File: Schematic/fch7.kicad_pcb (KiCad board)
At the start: 4 copper layers, 39.8 x 41.5 mm, 144 parts, among them IC1 MP9943AGQ-Z, IC2 MP9943AGQ-Z, IC4 ICM-42688-P, IC5 MPU-6500, J11 PIN2216, J12 PIN2216, J2 PIN2216, J3 PIN2216, J4 PIN2216, J5 PIN2216, J6 PIN2216, J7 PIN2216, J8 PIN2216, J9 PIN2216, U1 ME6217C33M5G, U10 HDGC1002WR-S-4P, U11 HDGC1002WR-S-4P, U12 E28-2G4M27SX, U13 STM32H742VIHx, U15 HDGC1002WR-S-6P, U16 HDGC1002WR-S-8P, U17 HDGC1002WR-S-8P, U2 ME6217C33M5G, U3 LDO-1.8v, U4 QMC5883L, U5 SPL06-001, U6 CSNP1GCR01-BOW, U7 HDGC1002WR-S-6P, U8 HDGC1002WR-S-4P, U9 HDGC1002WR-S-4P, Y1 8MHz

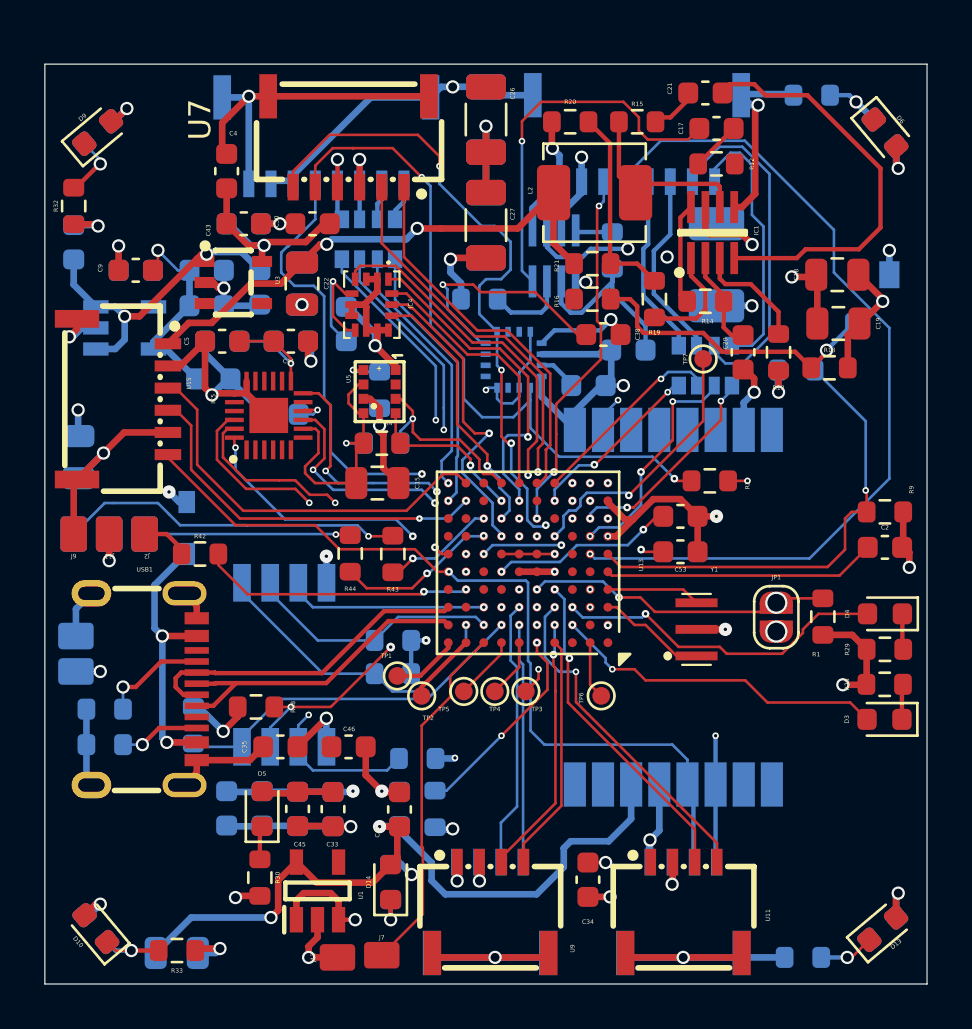
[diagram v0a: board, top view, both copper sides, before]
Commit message: update routing
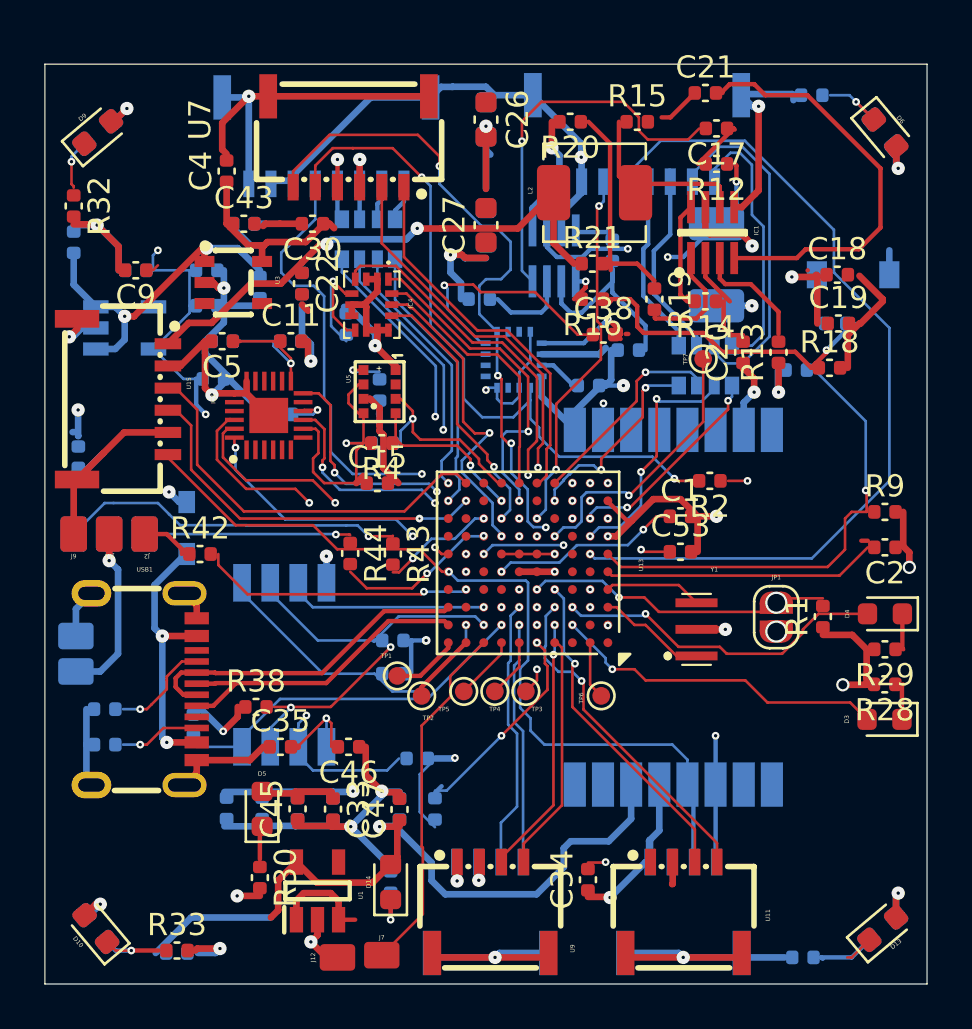
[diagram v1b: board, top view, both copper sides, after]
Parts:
- C1, C10, C11, C12, C14, C16, C17, C2, C20, C21, C28, C29, C3, C30, C31, C32, C33, C34, C35, C36, C37, C38, C39, C4, C40, C41, C43, C45, C46, C47, C5, C50, C53, C6, C7, C8, C9: footprint Capacitor_SMD:C_0603_1608Metric -> Capacitor_SMD:C_0402_1005Metric
- C13, C15, C18, C19, C22, C23, C48: footprint Capacitor_SMD:C_0805_2012Metric -> Capacitor_SMD:C_0402_1005Metric
- C24, C25, C26, C27: footprint Capacitor_SMD:C_1206_3216Metric -> Capacitor_SMD:C_0603_1608Metric
- R1, R10, R11, R12, R13, R14, R15, R16, R17, R18, R19, R2, R20, R21, R22, R28, R29, R3, R30, R31, R32, R33, R34, R35, R36, R37, R38, R39, R4, R40, R42, R43, R44, R5, R6, R7, R8, R9: footprint Resistor_SMD:R_0603_1608Metric -> Capacitor_SMD:C_0402_1005Metric
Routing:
- net GND: track 193.1 -> 207.8 mm, vias 38 -> 30
- net 5V: track 36.3 -> 43.5 mm, vias 15 -> 11
- net /Power/LC_5V: track 6.67 -> 12.6 mm, vias 2 -> 3
- net VDD_MCU: track 65.1 -> 71.0 mm
- net VBAT: track 26.9 -> 32.5 mm, vias 5 -> 4
- net Net-(D12-K): track 2.59 -> 3.92 mm, vias 1 -> 0
- net PWM_1: track 8.05 -> 9.23 mm
- net UART6_TX: track 24.3 -> 25.4 mm
- net Net-(D6-K): track 2.47 -> 3.56 mm
- net /Power/FB_5V: track 0.52 -> 1.58 mm
- net PWM_3: track 10.4 -> 11.0 mm
- net PWM_2: track 8.95 -> 9.48 mm
- net VDD_RECV: vias 2 -> 1
- net VCC_ICM: vias 2 -> 1
